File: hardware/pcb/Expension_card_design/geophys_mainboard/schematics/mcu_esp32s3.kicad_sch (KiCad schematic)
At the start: 13 parts, among them U4 74HC595D,118, U5 ESP32-S3-DevKitC, U6 74HC595D,118

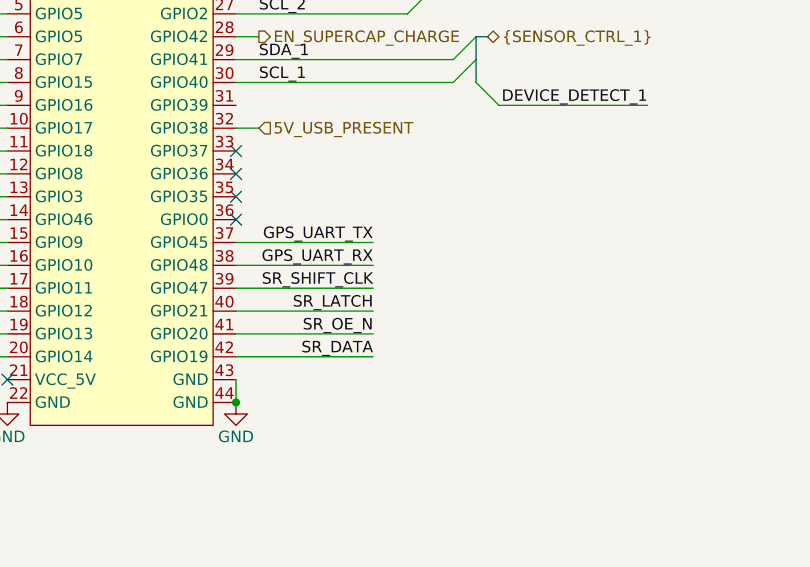
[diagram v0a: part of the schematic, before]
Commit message: ...
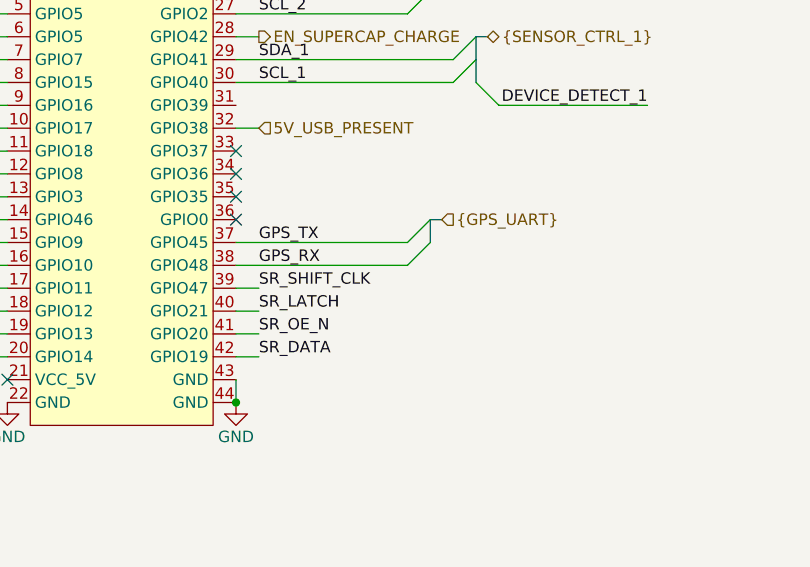
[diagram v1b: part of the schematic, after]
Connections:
- net GPS_UART_RX renamed GPS_RX
- net GPS_UART_TX renamed GPS_TX
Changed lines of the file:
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@@
 	(generator_version "9.0")
 	(paper "A3")
+	(bus_alias "GPS_UART"
+		(members "GPS_TX" "GPS_RX")
+	)
 	(bus_alias "SENSOR_CTRL_1"
 		(members "RESET_1" "SET_1" "SCL_1" "SDA_1" "DEVICE_DETECT_1")
@@
 	)
 	(bus_entry
+		(at 231.14 151.13)
+		(size -2.54 2.54)
+		(stroke
+			(width 0)
+			(type default)
+		)
+	)
+	(bus_entry
 		(at 149.86 158.75)
 		(size 2.54 2.54)
@@
 	)
 	(bus_entry
+		(at 231.14 148.59)
+		(size -2.54 2.54)
+		(stroke
+			(width 0)
+			(type default)
+		)
+	)
+	(bus_entry
 		(at 149.86 156.21)
 		(size 2.54 2.54)
@@
 	(bus
 		(pts
+			(xy 231.14 148.59) (xy 232.41 148.59)
+		)
+		(stroke
+			(width 0)
+			(type default)
+		)
+	)
+	(bus
+		(pts
 			(xy 158.75 138.43) (xy 158.75 146.05)
 		)
@@
 	(wire
 		(pts
-			(xy 224.79 151.13) (xy 209.55 151.13)
-		)
-		(stroke
-			(width 0)
-			(type default)
-		)
-	)
-	(wire
-		(pts
 			(xy 83.82 144.78) (xy 83.82 147.32)
 		)
@@
 	(wire
 		(pts
-			(xy 224.79 156.21) (xy 209.55 156.21)
-		)
-		(stroke
-			(width 0)
-			(type default)
-		)
-	)
-	(wire
-		(pts
 			(xy 93.98 167.64) (xy 106.68 167.64)
 		)
@@
 		)
 	)
-	(wire
-		(pts
-			(xy 224.79 158.75) (xy 209.55 158.75)
+	(bus
+		(pts
+			(xy 231.14 151.13) (xy 231.14 148.59)
+		)
+		(stroke
+			(width 0)
+			(type default)
+		)
+	)
+	(wire
+		(pts
+			(xy 212.09 158.75) (xy 209.55 158.75)
 		)
 		(stroke
@@
 	(wire
 		(pts
+			(xy 209.55 153.67) (xy 228.6 153.67)
+		)
+		(stroke
+			(width 0)
+			(type default)
+		)
+	)
+	(wire
+		(pts
 			(xy 161.29 148.59) (xy 184.15 148.59)
 		)
@@
 	(wire
 		(pts
+			(xy 209.55 151.13) (xy 228.6 151.13)
+		)
+		(stroke
+			(width 0)
+			(type default)
+		)
+	)
+	(wire
+		(pts
 			(xy 161.29 151.13) (xy 184.15 151.13)
 		)
@@
 	(wire
 		(pts
-			(xy 224.79 163.83) (xy 209.55 163.83)
+			(xy 212.09 163.83) (xy 209.55 163.83)
 		)
 		(stroke
@@
 	(wire
 		(pts
-			(xy 224.79 161.29) (xy 209.55 161.29)
+			(xy 212.09 161.29) (xy 209.55 161.29)
 		)
 		(stroke
@@
 	(wire
 		(pts
-			(xy 209.55 153.67) (xy 224.79 153.67)
-		)
-		(stroke
-			(width 0)
-			(type default)
-		)
-	)
-	(wire
-		(pts
 			(xy 54.61 157.48) (xy 73.66 157.48)
 		)
@@
 		(pts
 			(xy 168.91 158.75) (xy 184.15 158.75)
+		)
+		(stroke
+			(width 0)
+			(type default)
+		)
+	)
+	(wire
+		(pts
+			(xy 209.55 156.21) (xy 212.09 156.21)
 		)
 		(stroke
@@
 		)
 	)
-	(label "GPS_UART_TX"
-		(at 224.79 151.13 180)
-		(effects
-			(font
-				(size 1.27 1.27)
-			)
-			(justify right bottom)
-		)
-	)
 	(label "ESP_CS"
 		(at 181.61 156.21 180)
@@
 		)
 	)
+	(label "GPS_TX"
+		(at 212.09 151.13 0)
+		(effects
+			(font
+				(size 1.27 1.27)
+			)
+			(justify left bottom)
+		)
+	)
 	(label "SET_2"
 		(at 71.12 154.94 180)
@@
 		)
 	)
-	(label "GPS_UART_RX"
-		(at 224.79 153.67 180)
-		(effects
-			(font
-				(size 1.27 1.27)
-			)
-			(justify right bottom)
-		)
-	)
 	(label "MISO"
 		(at 181.61 151.13 180)
@@
 		)
 	)
+	(label "GPS_RX"
+		(at 212.09 153.67 0)
+		(effects
+			(font
+				(size 1.27 1.27)
+			)
+			(justify left bottom)
+		)
+	)
 	(label "ADC_START"
 		(at 71.12 160.02 180)
@@
 	)
 	(label "SR_OE_N"
-		(at 224.79 161.29 180)
-		(effects
-			(font
-				(size 1.27 1.27)
-			)
-			(justify right bottom)
+		(at 212.09 161.29 0)
+		(effects
+			(font
+				(size 1.27 1.27)
+			)
+			(justify left bottom)
 		)
 	)
@@
 	)
 	(label "SR_SHIFT_CLK"
-		(at 224.79 156.21 180)
-		(effects
-			(font
-				(size 1.27 1.27)
-			)
-			(justify right bottom)
+		(at 212.09 156.21 0)
+		(effects
+			(font
+				(size 1.27 1.27)
+			)
+			(justify left bottom)
 		)
 	)
@@
 	)
 	(label "SR_DATA"
-		(at 224.79 163.83 180)
-		(effects
-			(font
-				(size 1.27 1.27)
-			)
-			(justify right bottom)
+		(at 212.09 163.83 0)
+		(effects
+			(font
+				(size 1.27 1.27)
+			)
+			(justify left bottom)
 		)
 	)
@@
 	)
 	(label "SR_LATCH"
-		(at 224.79 158.75 180)
-		(effects
-			(font
-				(size 1.27 1.27)
-			)
-			(justify right bottom)
+		(at 212.09 158.75 0)
+		(effects
+			(font
+				(size 1.27 1.27)
+			)
+			(justify left bottom)
 		)
 	)
@@
 		)
 	)
+	(hierarchical_label "{GPS_UART}"
+		(shape input)
+		(at 232.41 148.59 0)
+		(effects
+			(font
+				(size 1.27 1.27)
+			)
+			(justify left)
+		)
+	)
